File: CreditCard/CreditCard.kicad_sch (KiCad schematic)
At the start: 9 parts

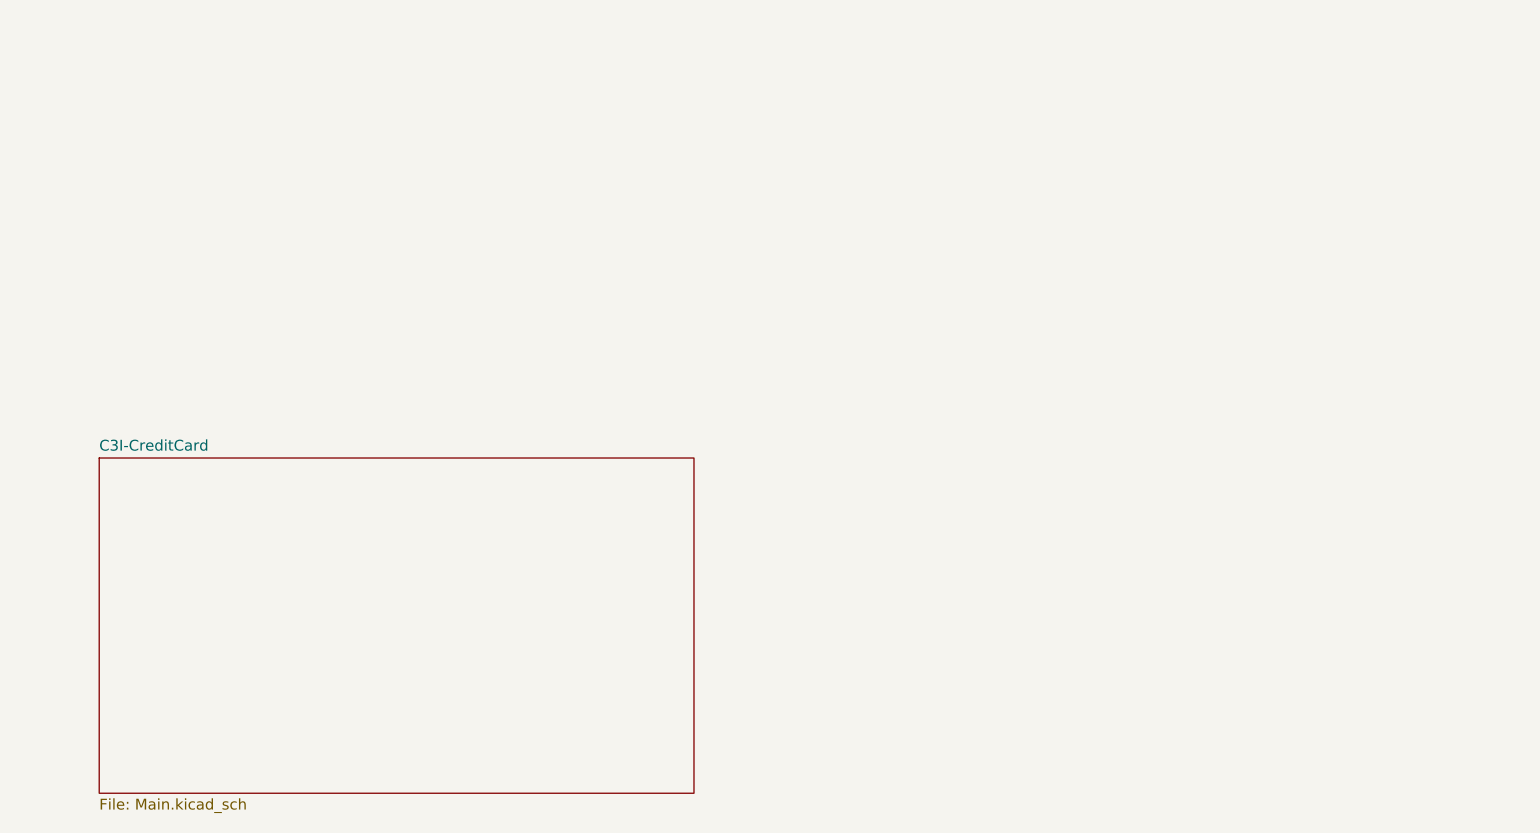
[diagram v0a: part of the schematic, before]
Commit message: début
début sch
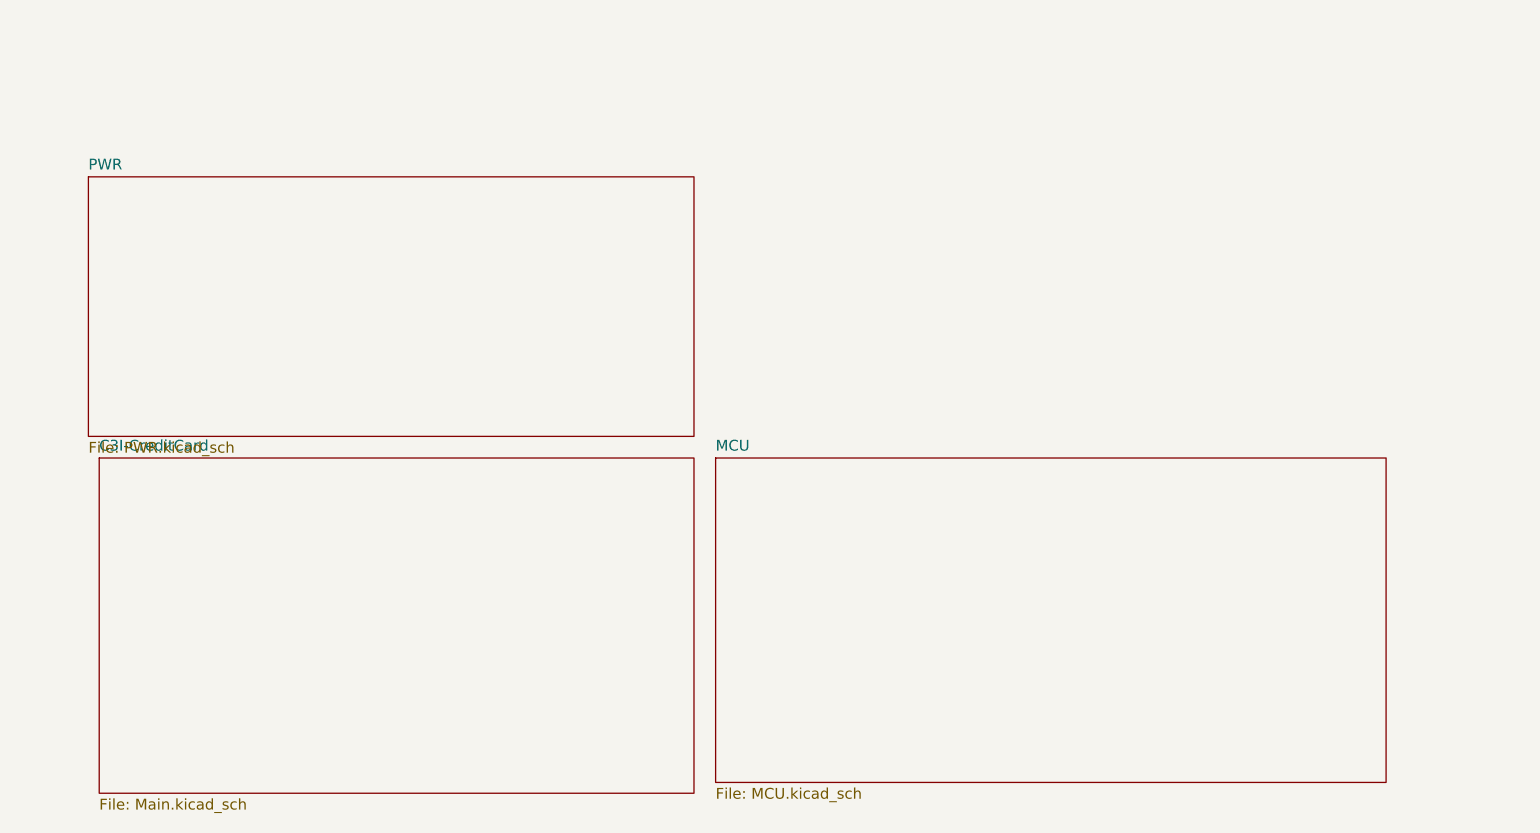
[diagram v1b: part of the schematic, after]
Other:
- added sheet MCU (MCU.kicad_sch)
- added sheet PWR (PWR.kicad_sch)
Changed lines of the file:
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@@
 (kicad_sch
-	(version 20231120)
+	(version 20250114)
 	(generator "eeschema")
-	(generator_version "8.0")
+	(generator_version "9.0")
 	(paper "A4")
+	(rectangle
+		(start 146.05 12.7)
+		(end 214.63 74.676)
+		(stroke
+			(width 0.381)
+			(type dash)
+			(color 20 0 0 1)
+		)
+		(fill
+			(type none)
+		)
+	)
+	(rectangle
+		(start 215.9 12.7)
+		(end 284.48 74.676)
+		(stroke
+			(width 0.381)
+			(type dash)
+			(color 20 0 0 1)
+		)
+		(fill
+			(type none)
+		)
+	)
+	(text "Équipe #10 - C3i\nPCB Carte de crédit\nA25"
+		(exclude_from_sim no)
+		(at 14.478 42.926 0)
+		(effects
+			(font
+				(face "Calibri")
+				(size 11.43 11.43)
+				(thickness 0.254)
+				(bold yes)
+			)
+			(justify left)
+		)
+	)
+	(text "BOTTOM\n"
+		(exclude_from_sim no)
+		(at 262.636 37.084 0)
+		(effects
+			(font
+				(size 2.286 2.286)
+				(thickness 0.4064)
+				(bold yes)
+			)
+		)
+	)
+	(text "TESTPOINTS"
+		(exclude_from_sim no)
+		(at 157.734 16.002 0)
+		(effects
+			(font
+				(size 2.286 2.286)
+				(thickness 0.4064)
+				(bold yes)
+			)
+		)
+	)
+	(text "FIDUCIALS\n"
+		(exclude_from_sim no)
+		(at 225.552 16.002 0)
+		(effects
+			(font
+				(size 2.286 2.286)
+				(thickness 0.4064)
+				(bold yes)
+			)
+		)
+	)
+	(text "TOP"
+		(exclude_from_sim no)
+		(at 236.474 37.592 0)
+		(effects
+			(font
+				(size 2.286 2.286)
+				(thickness 0.4064)
+				(bold yes)
+			)
+		)
+	)
 	(wire
 		(pts
@@
 		)
 	)
-	(rectangle
-		(start 146.05 12.7)
-		(end 214.63 74.676)
-		(stroke
-			(width 0.381)
-			(type dash)
-			(color 20 0 0 1)
-		)
-		(fill
-			(type none)
-		)
-	)
-	(rectangle
-		(start 215.9 12.7)
-		(end 284.48 74.676)
-		(stroke
-			(width 0.381)
-			(type dash)
-			(color 20 0 0 1)
-		)
-		(fill
-			(type none)
-		)
-	)
 	(image
 		(at 249.428 114.3)
@@
 		)
 	)
-	(text "Équipe #10 - C3i\nPCB Carte de crédit\nA25"
-		(exclude_from_sim no)
-		(at 14.478 42.926 0)
-		(effects
-			(font
-				(face "Calibri")
-				(size 11.43 11.43)
-				(thickness 0.254)
-				(bold yes)
-			)
-			(justify left)
-		)
-	)
-	(text "BOTTOM\n"
-		(exclude_from_sim no)
-		(at 262.636 37.084 0)
-		(effects
-			(font
-				(size 2.286 2.286)
-				(thickness 0.4064)
-				(bold yes)
-			)
-		)
-	)
-	(text "TESTPOINTS"
-		(exclude_from_sim no)
-		(at 157.734 16.002 0)
-		(effects
-			(font
-				(size 2.286 2.286)
-				(thickness 0.4064)
-				(bold yes)
-			)
-		)
-	)
-	(text "FIDUCIALS\n"
-		(exclude_from_sim no)
-		(at 225.552 16.002 0)
-		(effects
-			(font
-				(size 2.286 2.286)
-				(thickness 0.4064)
-				(bold yes)
-			)
-		)
-	)
-	(text "TOP"
-		(exclude_from_sim no)
-		(at 236.474 37.592 0)
-		(effects
-			(font
-				(size 2.286 2.286)
-				(thickness 0.4064)
-				(bold yes)
-			)
-		)
-	)
 	(symbol
 		(lib_id "LIB:Fiducial")
@@
 		(at 24.13 144.78)
 		(size 69.85 39.37)
+		(exclude_from_sim no)
+		(in_bom yes)
+		(on_board yes)
+		(dnp no)
 		(fields_autoplaced yes)
 		(stroke
@@
 		)
 	)
+	(sheet
+		(at 22.86 111.76)
+		(size 71.12 30.48)
+		(exclude_from_sim no)
+		(in_bom yes)
+		(on_board yes)
+		(dnp no)
+		(fields_autoplaced yes)
+		(stroke
+			(width 0.1524)
+			(type solid)
+		)
+		(fill
+			(color 0 0 0 0.0000)
+		)
+		(property "Sheetname" "PWR"
+			(at 22.86 111.0484 0)
+			(effects
+				(font
+					(size 1.27 1.27)
+				)
+				(justify left bottom)
+			)
+		)
+		(property "Sheetfile" "PWR.kicad_sch"
+			(at 22.86 142.8246 0)
+			(effects
+				(font
+					(size 1.27 1.27)
+				)
+				(justify left top)
+			)
+		)
+		(instances
+			(project "CreditCard"
+				(path "/374dba13-75d6-44a0-b8b2-0ca0aa70330e"
+					(page "4")
+				)
+			)
+		)
+	)
+	(sheet
+		(at 96.52 144.78)
+		(size 78.74 38.1)
+		(exclude_from_sim no)
+		(in_bom yes)
+		(on_board yes)
+		(dnp no)
+		(fields_autoplaced yes)
+		(stroke
+			(width 0.1524)
+			(type solid)
+		)
+		(fill
+			(color 0 0 0 0.0000)
+		)
+		(property "Sheetname" "MCU"
+			(at 96.52 144.0684 0)
+			(effects
+				(font
+					(size 1.27 1.27)
+				)
+				(justify left bottom)
+			)
+		)
+		(property "Sheetfile" "MCU.kicad_sch"
+			(at 96.52 183.4646 0)
+			(effects
+				(font
+					(size 1.27 1.27)
+				)
+				(justify left top)
+			)
+		)
+		(instances
+			(project "CreditCard"
+				(path "/374dba13-75d6-44a0-b8b2-0ca0aa70330e"
+					(page "3")
+				)
+			)
+		)
+	)
 	(sheet_instances
 		(path "/"
@@
 		)
 	)
+	(embedded_fonts no)
 )
